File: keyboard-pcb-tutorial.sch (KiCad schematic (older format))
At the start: 24 parts, among them SW1 SW_Push, U1 ATmega32U4-AU, Y1 16MHz

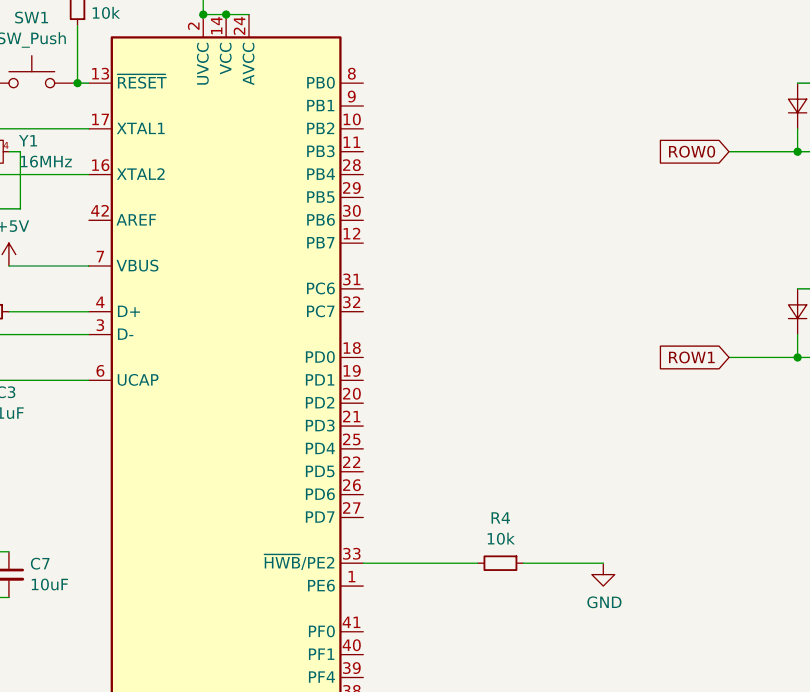
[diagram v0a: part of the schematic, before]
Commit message: Finished routing
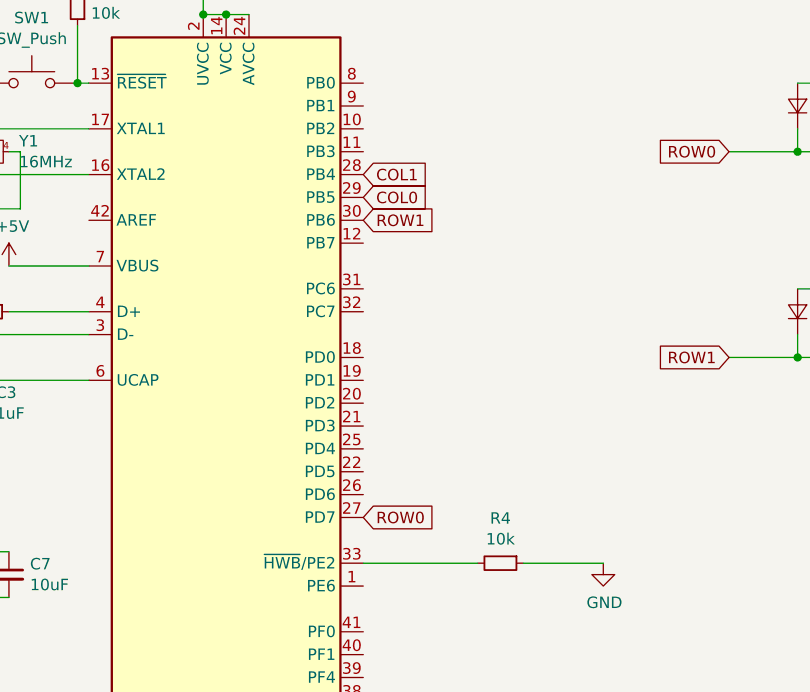
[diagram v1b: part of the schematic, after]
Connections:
- net COL0: now also U1.29 (PB5)
- net COL1: now also U1.28 (PB4)
- net ROW0: now also U1.27 (PD7)
- net ROW1: now also U1.30 (PB6)
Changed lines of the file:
@@
 Text GLabel 7900 1200 1    50   Input ~ 0
 COL1
+Text GLabel 4600 3600 2    50   Input ~ 0
+ROW0
+Text GLabel 4600 2300 2    50   Input ~ 0
+ROW1
+Text GLabel 4600 2200 2    50   Input ~ 0
+COL0
+Text GLabel 4600 2100 2    50   Input ~ 0
+COL1
 $EndSCHEMATC
